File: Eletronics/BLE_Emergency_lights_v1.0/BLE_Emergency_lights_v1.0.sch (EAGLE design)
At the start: 167 parts, among them IC1 SI7021-, U1 LIS2DH12

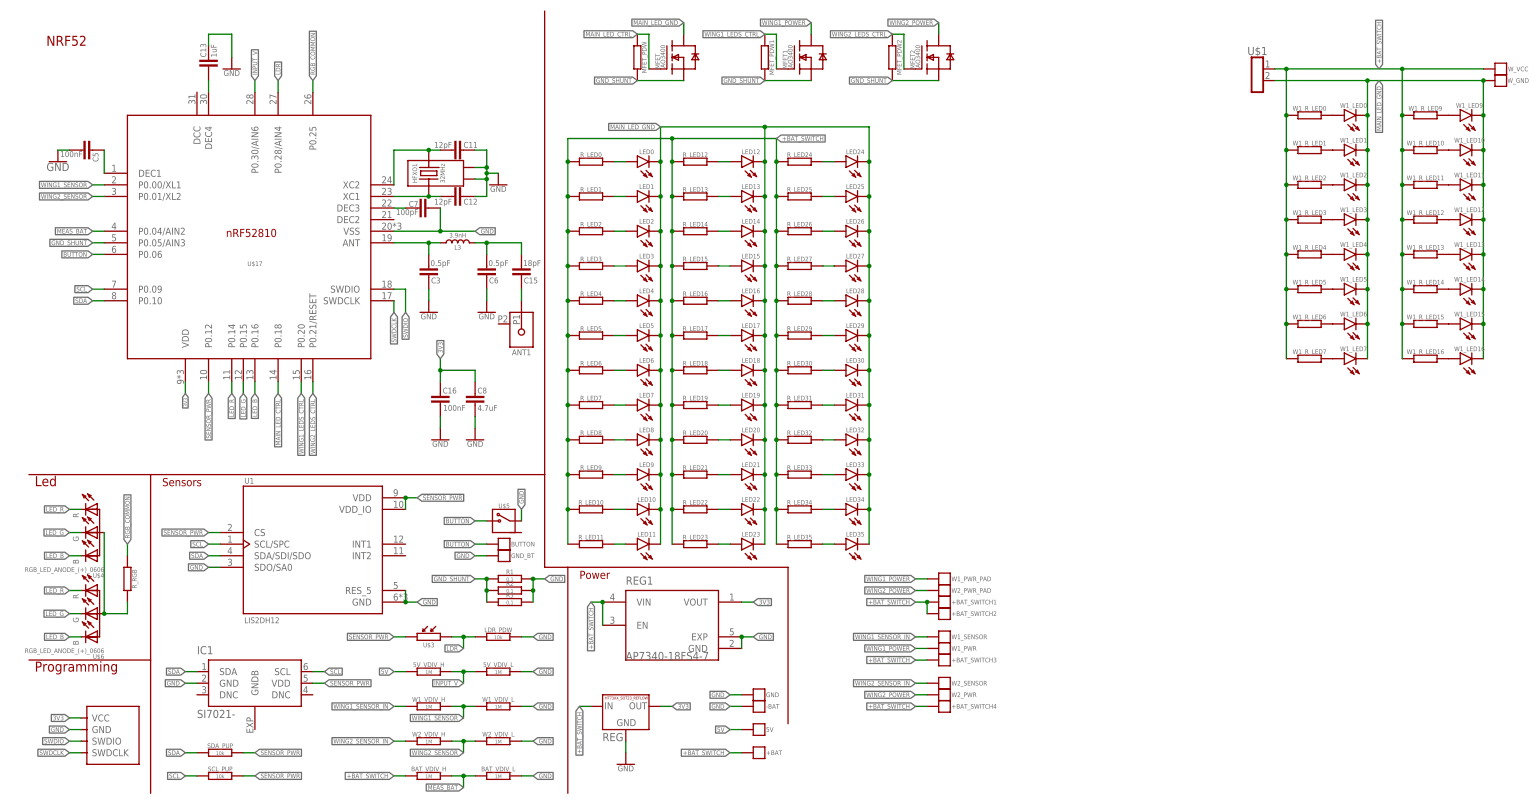
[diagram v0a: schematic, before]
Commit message: BLE_Emergency_lights_v1.0
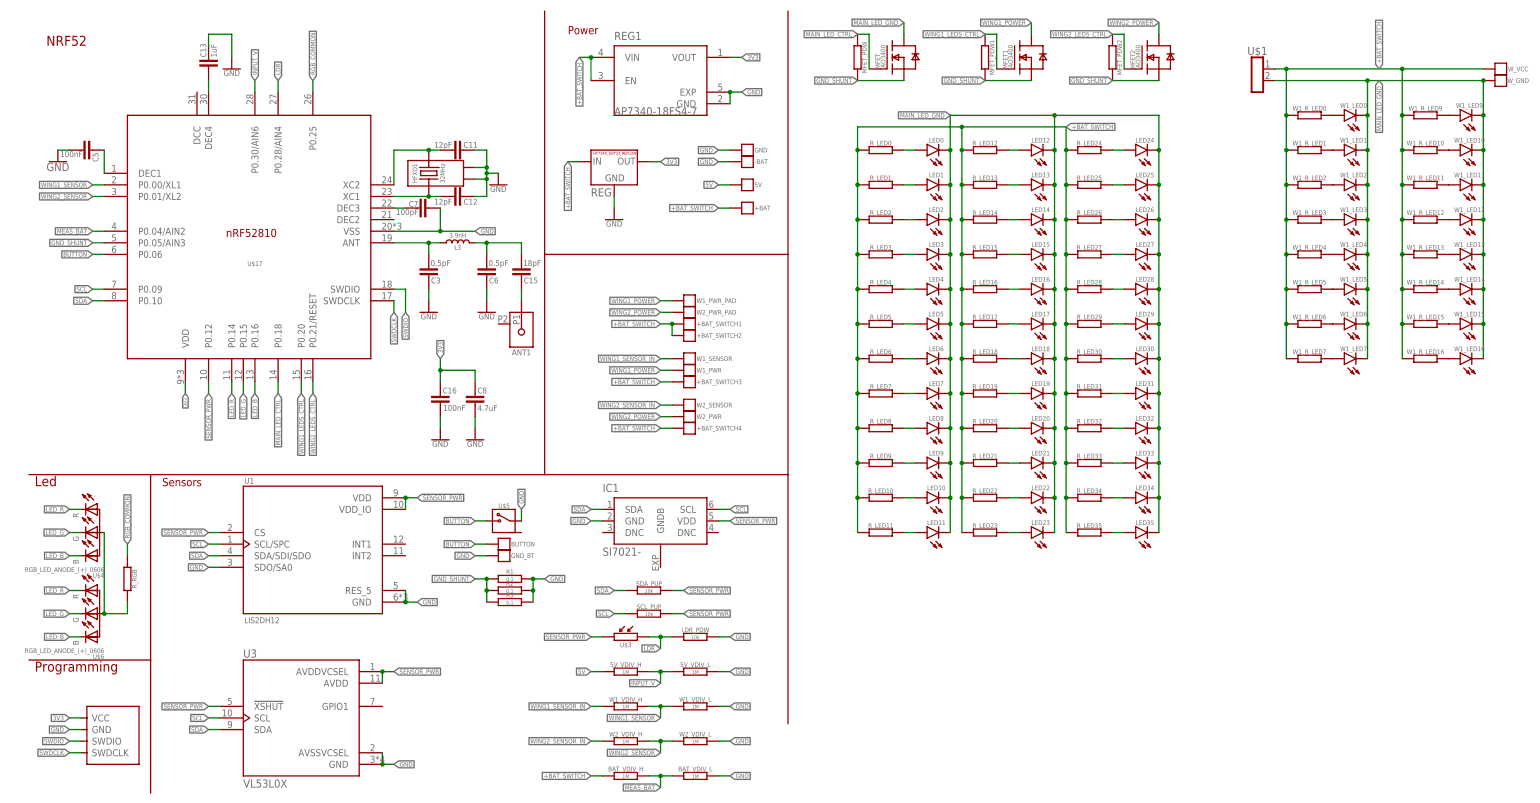
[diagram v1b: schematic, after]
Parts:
- added U3: VL53L0X, 0000_GV_sensors:VL53L0X
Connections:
- net GND: now also U3.AVSSVCSEL, U3.GND
- net SCL: now also U3.SCL
- net SDA: now also U3.SDA
- net SENSOR_PWR: now also U3.!XSHUT, U3.AVDD, U3.AVDDVCSEL
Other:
- moved on the sheet: +BAT, +BAT_SWITCH1, +BAT_SWITCH2, +BAT_SWITCH3, +BAT_SWITCH4, -BAT, 5V, 5V_VDIV_H, 5V_VDIV_L, BAT_VDIV_H, BAT_VDIV_L, GND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
